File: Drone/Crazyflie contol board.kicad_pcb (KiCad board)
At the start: 2 copper layers, 23 x 40 mm, 14 parts, among them J1 Aux, J2 Motors, J3 Conn_01x05_Pin, U2 BMP388, U3 BNO055

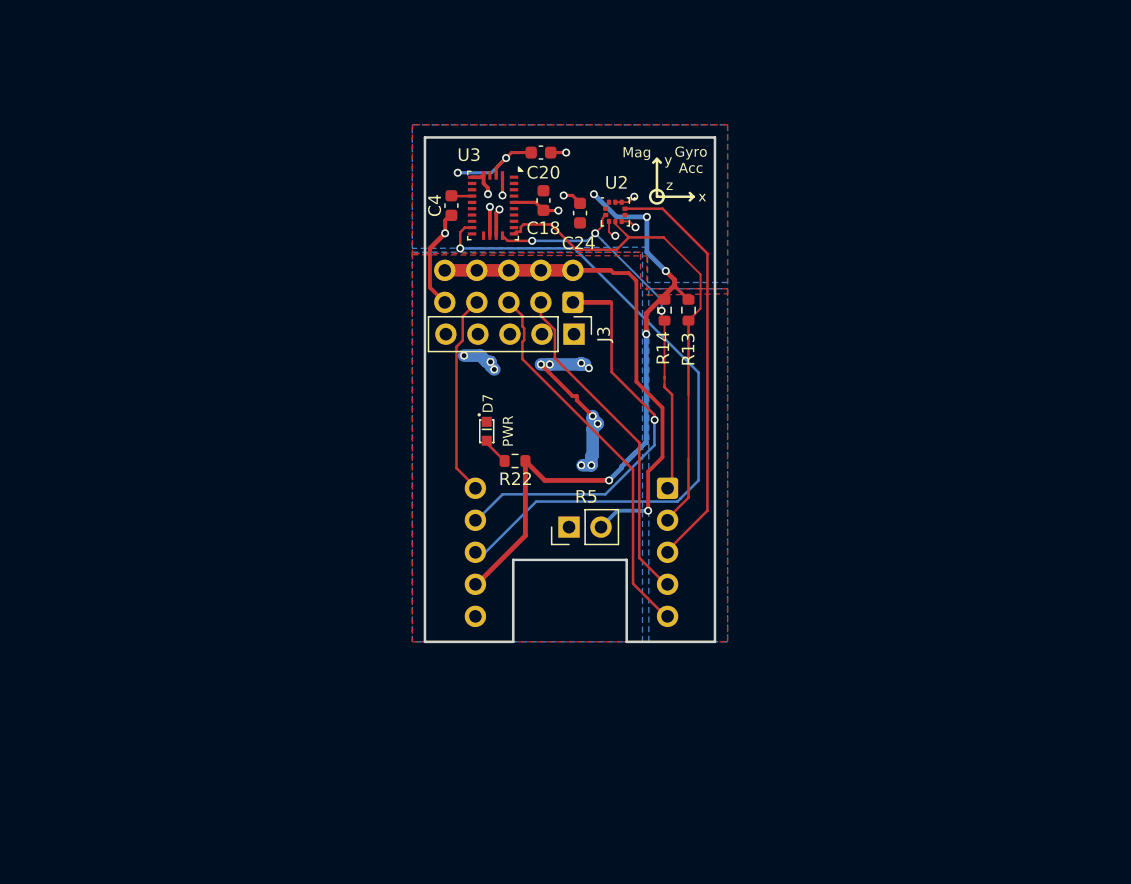
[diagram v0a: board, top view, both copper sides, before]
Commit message: save
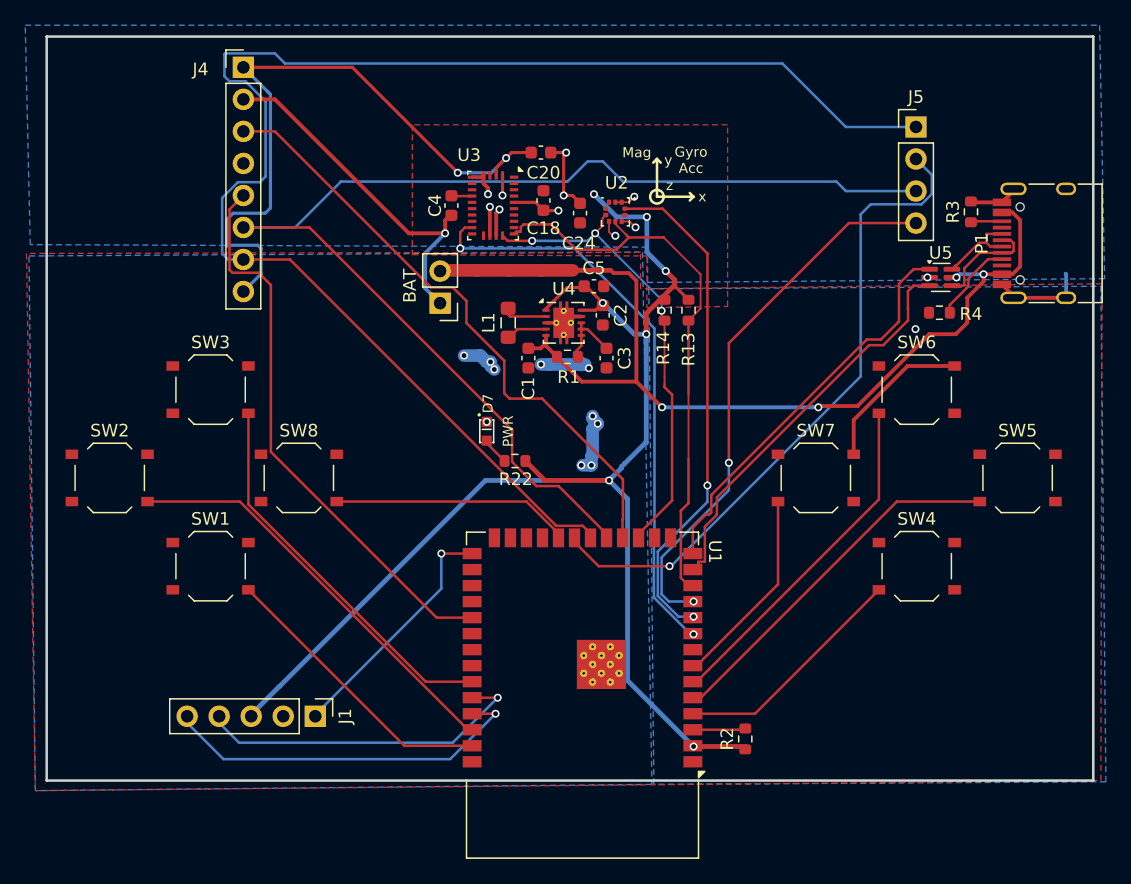
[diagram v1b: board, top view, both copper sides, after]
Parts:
- removed J2: Motors, Connector_IDC:IDC-Header_2x05_P2.54mm_Vertical
- removed J3: Conn_01x05_Pin, Connector_PinHeader_2.54mm:PinHeader_1x05_P2.54mm_Vertical
- added C1: 10uF, Capacitor_SMD:C_0603_1608Metric, F.Cu at (134.2, 100.5)
- added C2: 10uF, Capacitor_SMD:C_0603_1608Metric, F.Cu at (140.1, 97.1)
- added C3: 100nF, Capacitor_SMD:C_0603_1608Metric, F.Cu at (140.4, 100.5)
- added C5: 10uF, Capacitor_SMD:C_0603_1608Metric, F.Cu at (139.4, 94.8)
- added J4: Conn_01x08_Pin, Connector_PinHeader_2.54mm:PinHeader_1x08_P2.54mm_Vertical, F.Cu at (111.6, 77.4)
- added J5: Conn_01x04_Pin, Connector_PinHeader_2.54mm:PinHeader_1x04_P2.54mm_Vertical, F.Cu at (164.9, 82.2)
- added L1: 2.2uH, Inductor_SMD:L_0805_2012Metric_Pad1.05x1.20mm_HandSolder, F.Cu at (132.6, 97.7)
- added P1: USB_C_Plug_USB2.0, Connector_USB:USB_C_Receptacle_HRO_TYPE-C-31-M-12, F.Cu at (175.8, 91.4)
- added R1: 100R, Resistor_SMD:R_0603_1608Metric, F.Cu at (137.3, 100.4)
- added R2: 10k, Resistor_SMD:R_0603_1608Metric, F.Cu at (151.4, 130.7)
- added R3: 5.1k, Resistor_SMD:R_0603_1608Metric, F.Cu at (169.3, 88.9)
- added R4: 5.1k, Resistor_SMD:R_0603_1608Metric, F.Cu at (166.8, 96.9)
- added SW1: SW_Push, Button_Switch_SMD:SW_Push_1P1T_XKB_TS-1187A, F.Cu at (109.0, 117.0)
- added SW2: SW_Push, Button_Switch_SMD:SW_Push_1P1T_XKB_TS-1187A, F.Cu at (101.0, 110.0)
- added SW3: SW_Push, Button_Switch_SMD:SW_Push_1P1T_XKB_TS-1187A, F.Cu at (109.0, 103.0)
- added SW4: SW_Push, Button_Switch_SMD:SW_Push_1P1T_XKB_TS-1187A, F.Cu at (165.0, 117.0)
- added SW5: SW_Push, Button_Switch_SMD:SW_Push_1P1T_XKB_TS-1187A, F.Cu at (173.0, 110.0)
- added SW6: SW_Push, Button_Switch_SMD:SW_Push_1P1T_XKB_TS-1187A, F.Cu at (165.0, 103.0)
- added SW7: SW_Push, Button_Switch_SMD:SW_Push_1P1T_XKB_TS-1187A, F.Cu at (157.0, 110.0)
- added SW8: SW_Push, Button_Switch_SMD:SW_Push_1P1T_XKB_TS-1187A, F.Cu at (116.0, 110.0)
- added U1: ESP32-S3-WROOM-1, RF_Module:ESP32-S3-WROOM-1, F.Cu at (138.5, 127.2)
- added U4: TPS63000, Package_SON:Texas_DRC0010J_ThermalVias, F.Cu at (137.0, 97.7)
- added U5: NUF2221-Crazyflie-contol-board-rescue, Package_TO_SOT_SMD:SOT-363_SC-70-6, F.Cu at (166.9, 94.1)
- J1: value Aux -> Conn_01x05_Pin; footprint Connector_IDC:IDC-Header_2x05_P2.54mm_Vertical -> Connector_PinHeader_2.54mm:PinHeader_1x05_P2.54mm_Vertical; moved to F.Cu
- moved J1 23.6 mm to (117.3, 128.9), turned to -90 degrees
- moved BAT 20.5 mm to (127.2, 96.1), turned to 180 degrees
- renumbered R5 to BAT
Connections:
- J1 pad 1: /I2C_SCL -> INT0
- J1 pad 2: M4 -> GND
- J1 pad 3: /I2C_SDA -> VCC
- J1 pad 4: M1 -> /RX
- J1 pad 5: INT3 -> /TX
- U2 pad 7: INT3 -> INT2
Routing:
- net /SCK: track 0.00 -> 116.4 mm
- net VCC: track 58.6 -> 167.6 mm, vias 7 -> 9
- net /MOSI: track 0.00 -> 97.1 mm
- net /MISO: track 0.00 -> 52.5 mm, vias 0 -> 1
- net /CS2: track 0.00 -> 48.7 mm
- net /DC: track 0.00 -> 44.8 mm
- net GND: track 46.0 -> 90.2 mm, vias 22 -> 23
- net /CS1: track 0.00 -> 43.7 mm, vias 0 -> 2
- net /USBD-: track 0.00 -> 40.4 mm
- net INT2: track 0.00 -> 40.3 mm, vias 0 -> 2
- net +BATT: track 39.4 -> 79.1 mm, vias 1 -> 4
- net /USBD+: track 0.00 -> 38.8 mm
- net Net-(U1-IO2): track 0.00 -> 33.2 mm
- net INT3: track 33.1 -> 0.00 mm
- net M1: track 32.3 -> 0.00 mm, vias 1 -> 0
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- removed copper zone on B.Cu, net +BATT
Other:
- board size 23 x 40 mm -> 83 x 59 mm
- board text added: "Rev. 1.0"
- board text removed: "Rev. 2.4"
